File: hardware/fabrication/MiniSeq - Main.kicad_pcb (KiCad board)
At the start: 2 copper layers, 170 x 128.5 mm, 97 parts, among them J1 Conn_01x10_Pin, SW1 SMTS-102, SW11 RESET_BTN, SW2 SMTS-102, SW3 SMTS-102, SW4 SMTS-102, SW5 SMTS-102, SW6 SMTS-102, SW7 SMTS-102, SW8 SMTS-102, SW9 CLOCK_BTN, U1 4017, U2 TL072, U3 TL074, U4 L7809CD2T-TR

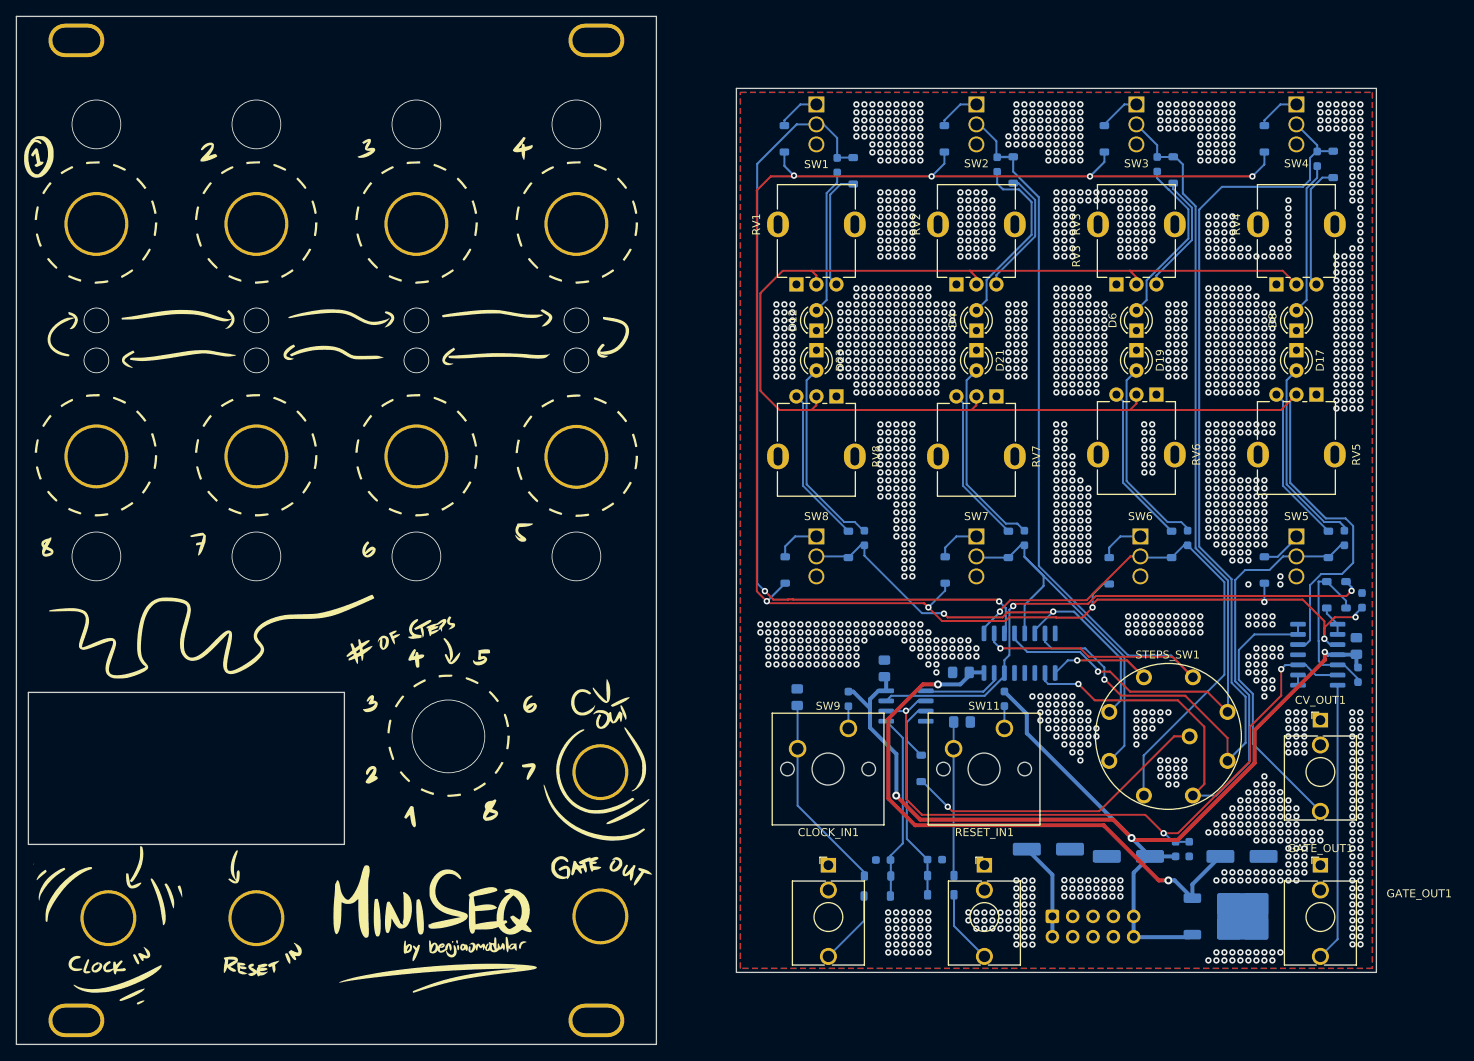
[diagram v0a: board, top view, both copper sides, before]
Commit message: v0.1 PCBs
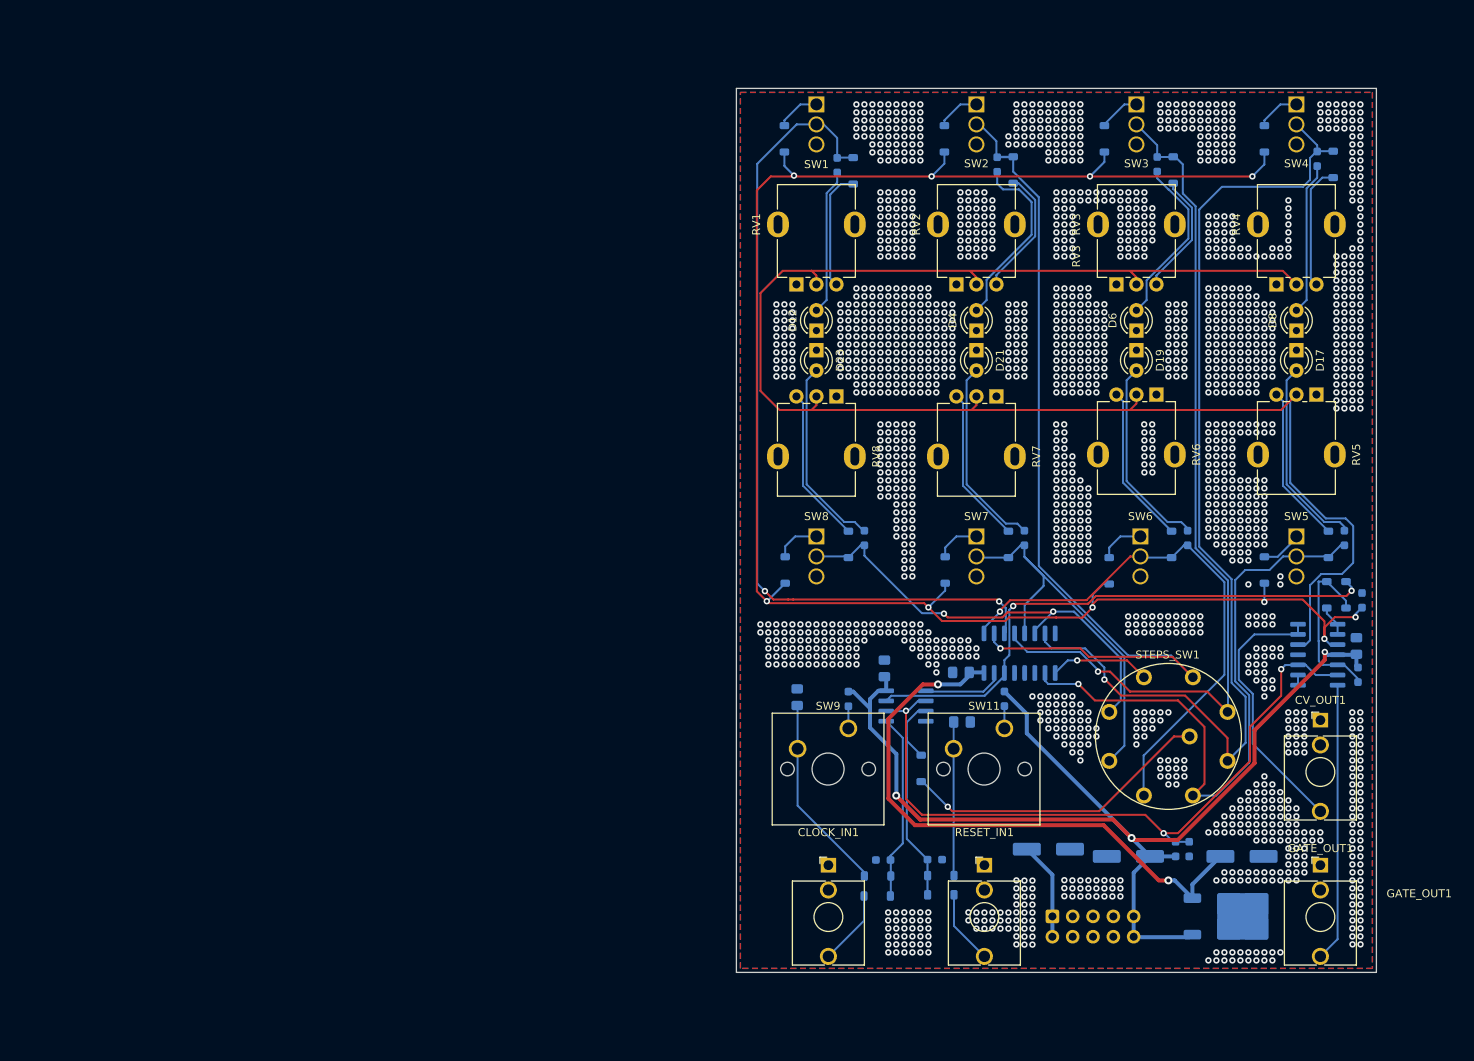
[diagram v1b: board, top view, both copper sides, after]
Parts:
- removed G***: LOGO, LOGO
- removed REF** (x8): PanelHole_Potentiometer_RV09, benjiaomodular:PanelHole_Potentiometer_RV09
- removed REF** (x4): PanelHole_AudioJack_3.5mm, benjiaomodular:PanelHole_AudioJack_3.5mm
- removed REF**: Panel_16HP, benjiaomodular:Panel_16HP
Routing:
- net (no net): vias 17 -> 0
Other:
- board size 170 x 128.5 mm -> 80 x 110.5 mm
